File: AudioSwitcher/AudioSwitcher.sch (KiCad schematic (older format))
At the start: 18 parts

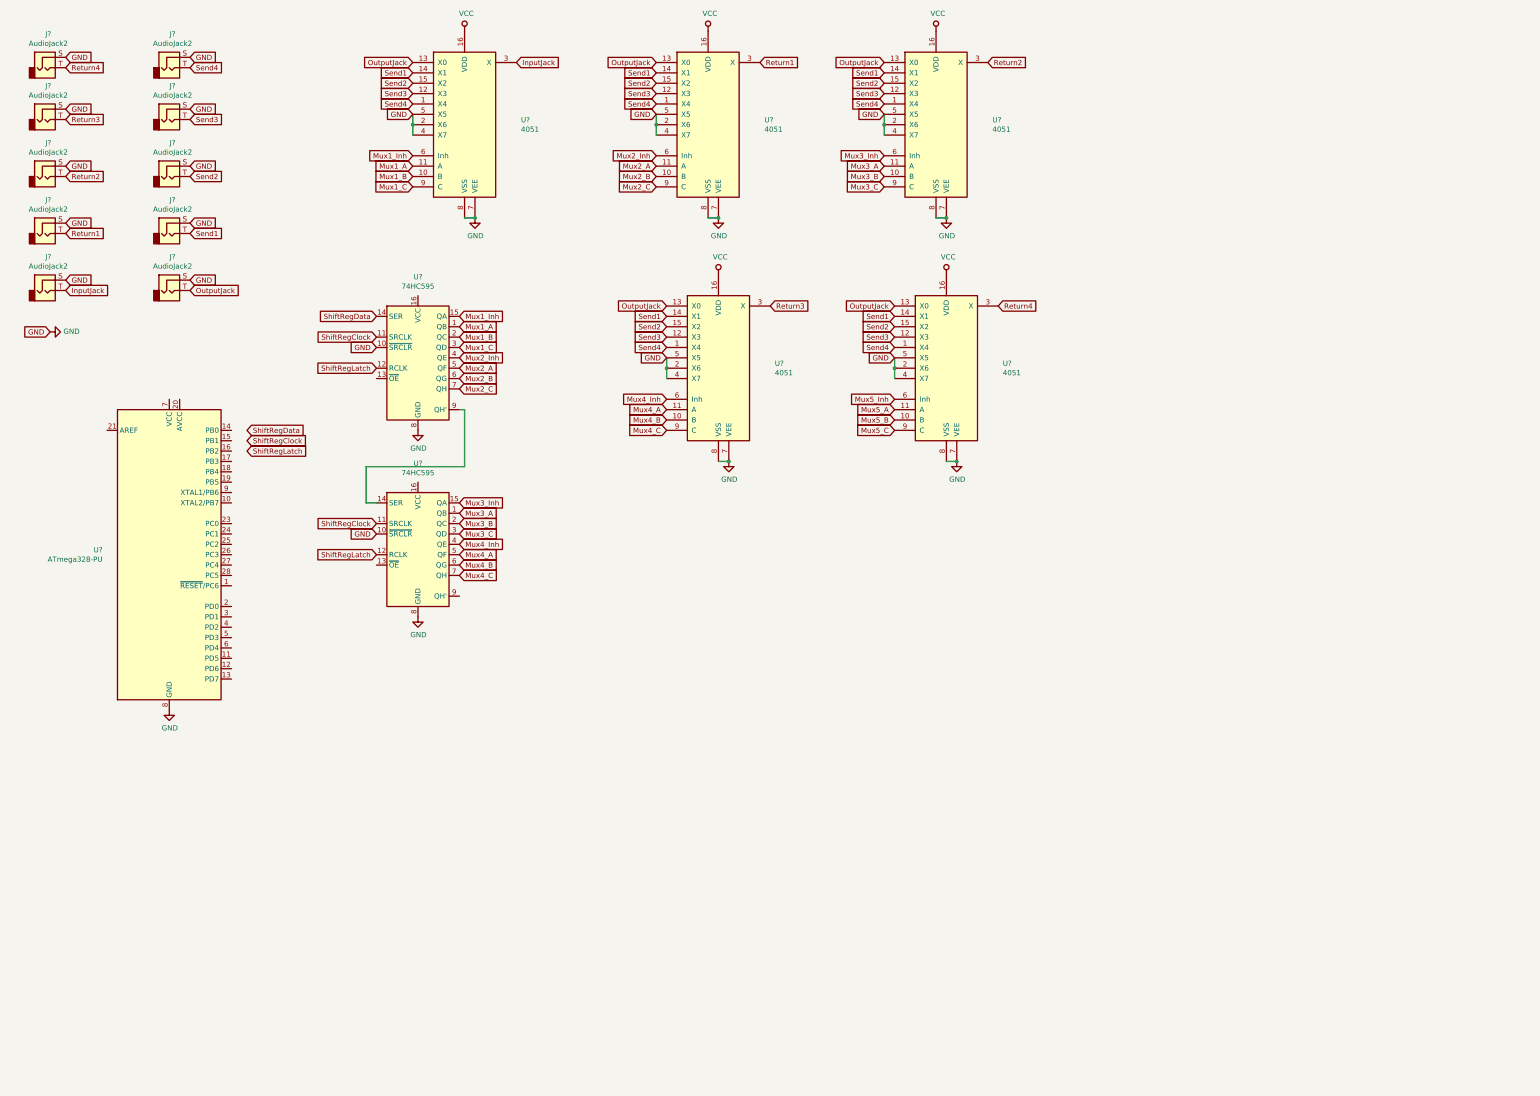
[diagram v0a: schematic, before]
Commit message: Updated schematic
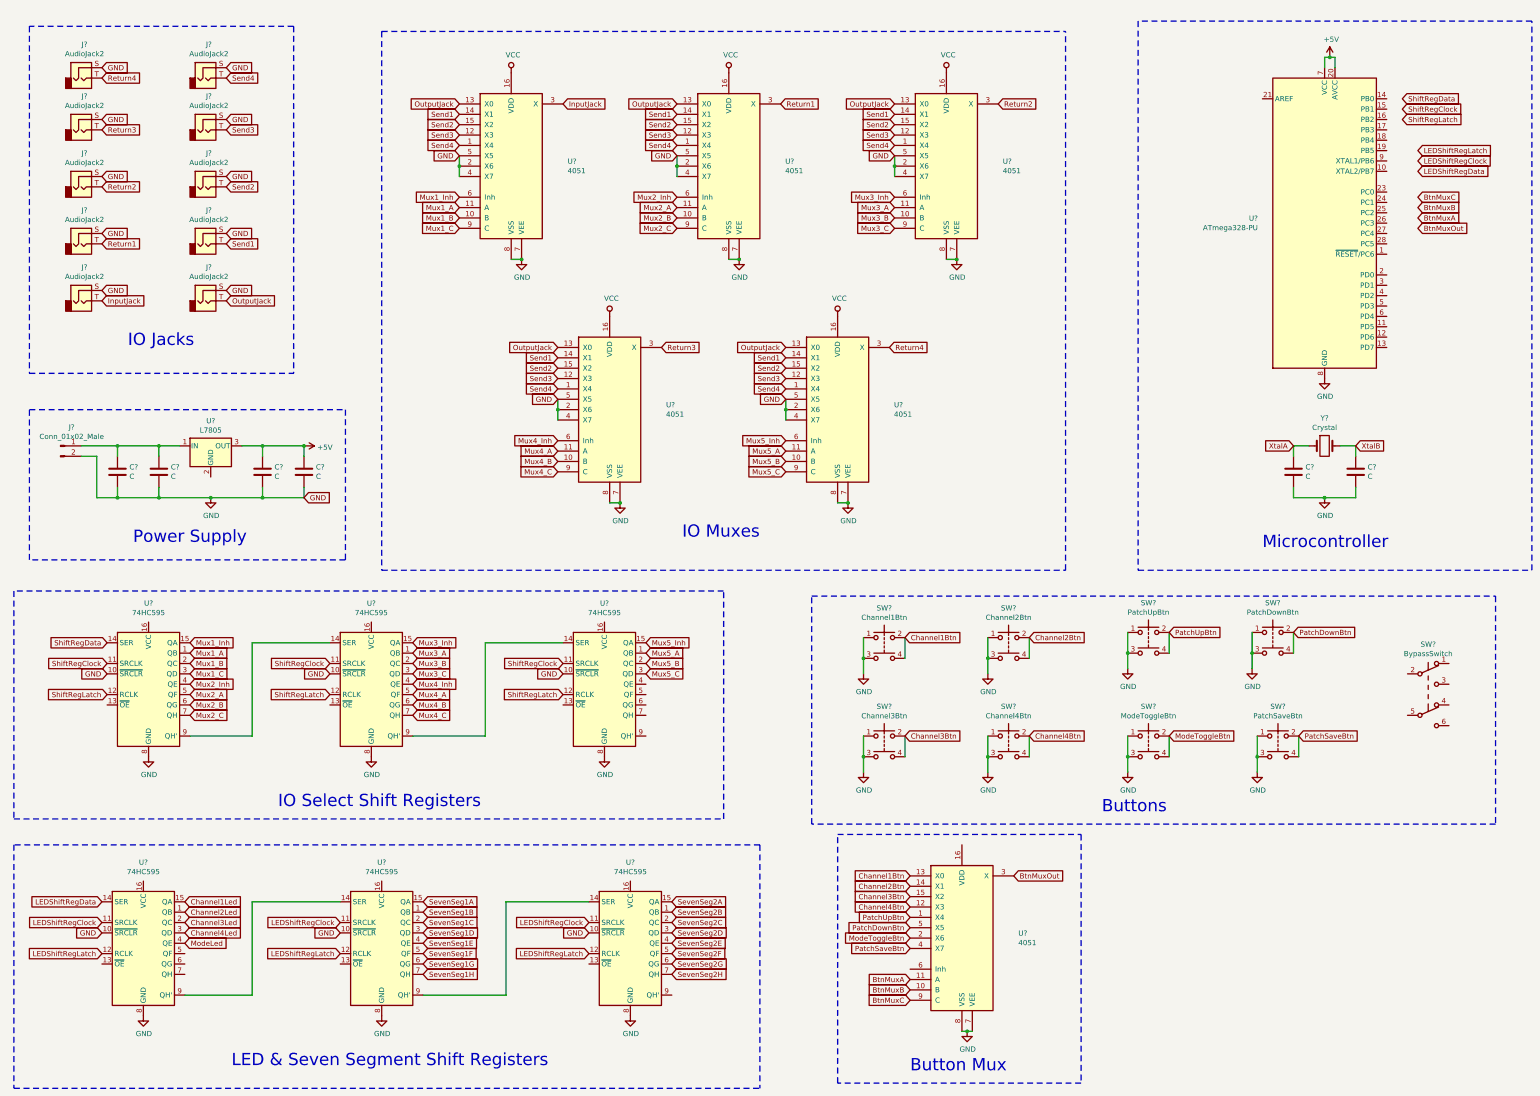
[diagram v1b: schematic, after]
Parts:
- added C? (x6): C, symbol Device:C
- added J?: Conn_01x02_Male, symbol Connector:Conn_01x02_Male
- added SW?: Channel1Btn, symbol Switch:SW_Push_Dual
- added SW?: Channel2Btn, symbol Switch:SW_Push_Dual
- added SW?: Channel3Btn, symbol Switch:SW_Push_Dual
- added SW?: Channel4Btn, symbol Switch:SW_Push_Dual
- added SW?: PatchUpBtn, symbol Switch:SW_Push_Dual
- added SW?: PatchDownBtn, symbol Switch:SW_Push_Dual
- added SW?: ModeToggleBtn, symbol Switch:SW_Push_Dual
- added SW?: PatchSaveBtn, symbol Switch:SW_Push_Dual
- added SW?: BypassSwitch, symbol Switch:SW_Push_DPDT
- added U? (x4): 74HC595, symbol 74xx:74HC595
- added U?: 4051, symbol 4xxx:4051
- added U?: L7805, symbol Regulator_Linear:L7805
- added Y?: Crystal, symbol Device:Crystal
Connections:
- net GND: now also C?.2, C?.2, C?.2, C?.2, C?.2, C?.2, J?.2 (Pin_2), SW?.1, SW?.1, SW?.1, SW?.1, SW?.1, SW?.1, SW?.1, SW?.1, SW?.3, SW?.3, SW?.3, SW?.3, SW?.3, SW?.3, SW?.3, SW?.3, U?.10 (~SRCLR), U?.10 (~SRCLR), U?.10 (~SRCLR), U?.10 (~SRCLR), U?.7 (VEE), U?.8 (GND), U?.8 (GND), U?.8 (GND), U?.8 (GND), U?.8 (VSS)
- net Mux5_A: now also U?.1 (QB)
- net Mux5_B: now also U?.2 (QC)
- net Mux5_C: now also U?.3 (QD)
- net Mux5_Inh: now also U?.15 (QA)
- net ShiftRegClock: now also U?.11 (SRCLK)
- net ShiftRegLatch: now also U?.12 (RCLK)
- net +5V: now reaches U?.20 (AVCC)
- net +5V: now also U?.7 (VCC), C?.1, C?.1, U?.3 (OUT)
- net at U?.9 (QH'): now also U?.14 (SER)
- new net: U?.14 (SER), U?.9 (QH') (x2)
- new net: C?.1, C?.1, J?.1 (Pin_1), U?.1 (IN)
- new net BtnMuxA: U?.11 (A)
- new net BtnMuxB: U?.10 (B)
- new net BtnMuxC: U?.9 (C)
- new net BtnMuxOut: U?.3 (X)
- new net Channel1Btn: SW?.2, SW?.4, U?.13 (X0)
- new net Channel1Led: U?.15 (QA)
- new net Channel2Btn: SW?.2, SW?.4, U?.14 (X1)
- new net Channel2Led: U?.1 (QB)
- new net Channel3Btn: SW?.2, SW?.4, U?.15 (X2)
- new net Channel3Led: U?.2 (QC)
- new net Channel4Btn: SW?.2, SW?.4, U?.12 (X3)
- new net Channel4Led: U?.3 (QD)
- new net LEDShiftRegClock: U?.11 (SRCLK), U?.11 (SRCLK), U?.11 (SRCLK)
- new net LEDShiftRegData: U?.14 (SER)
- new net LEDShiftRegLatch: U?.12 (RCLK), U?.12 (RCLK), U?.12 (RCLK)
- new net ModeLed: U?.4 (QE)
- new net ModeToggleBtn: SW?.2, SW?.4, U?.2 (X6)
- new net PatchDownBtn: SW?.2, SW?.4, U?.5 (X5)
- new net PatchSaveBtn: SW?.2, SW?.4, U?.4 (X7)
- new net PatchUpBtn: SW?.2, SW?.4, U?.1 (X4)
- new net SevenSeg1A: U?.15 (QA)
- new net SevenSeg1B: U?.1 (QB)
- new net SevenSeg1C: U?.2 (QC)
- new net SevenSeg1D: U?.3 (QD)
- new net SevenSeg1E: U?.4 (QE)
- new net SevenSeg1F: U?.5 (QF)
- new net SevenSeg1G: U?.6 (QG)
- new net SevenSeg1H: U?.7 (QH)
- new net SevenSeg2A: U?.15 (QA)
- new net SevenSeg2B: U?.1 (QB)
- new net SevenSeg2C: U?.2 (QC)
- new net SevenSeg2D: U?.3 (QD)
- new net SevenSeg2E: U?.4 (QE)
- new net SevenSeg2F: U?.5 (QF)
- new net SevenSeg2G: U?.6 (QG)
- new net SevenSeg2H: U?.7 (QH)
- new net XtalA: C?.1, Y?.1
- new net XtalB: C?.1, Y?.2
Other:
- note added: "Button Mux"
- note added: "Buttons"
- note added: "IO Jacks\n"
- note added: "IO Muxes"
- note added: "IO Select Shift Registers"
- note added: "LED & Seven Segment Shift Registers"
- note added: "Microcontroller"
- note added: "Power Supply"
- moved on the sheet: J?, U?
